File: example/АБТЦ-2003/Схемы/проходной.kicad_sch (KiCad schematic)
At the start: 27 parts

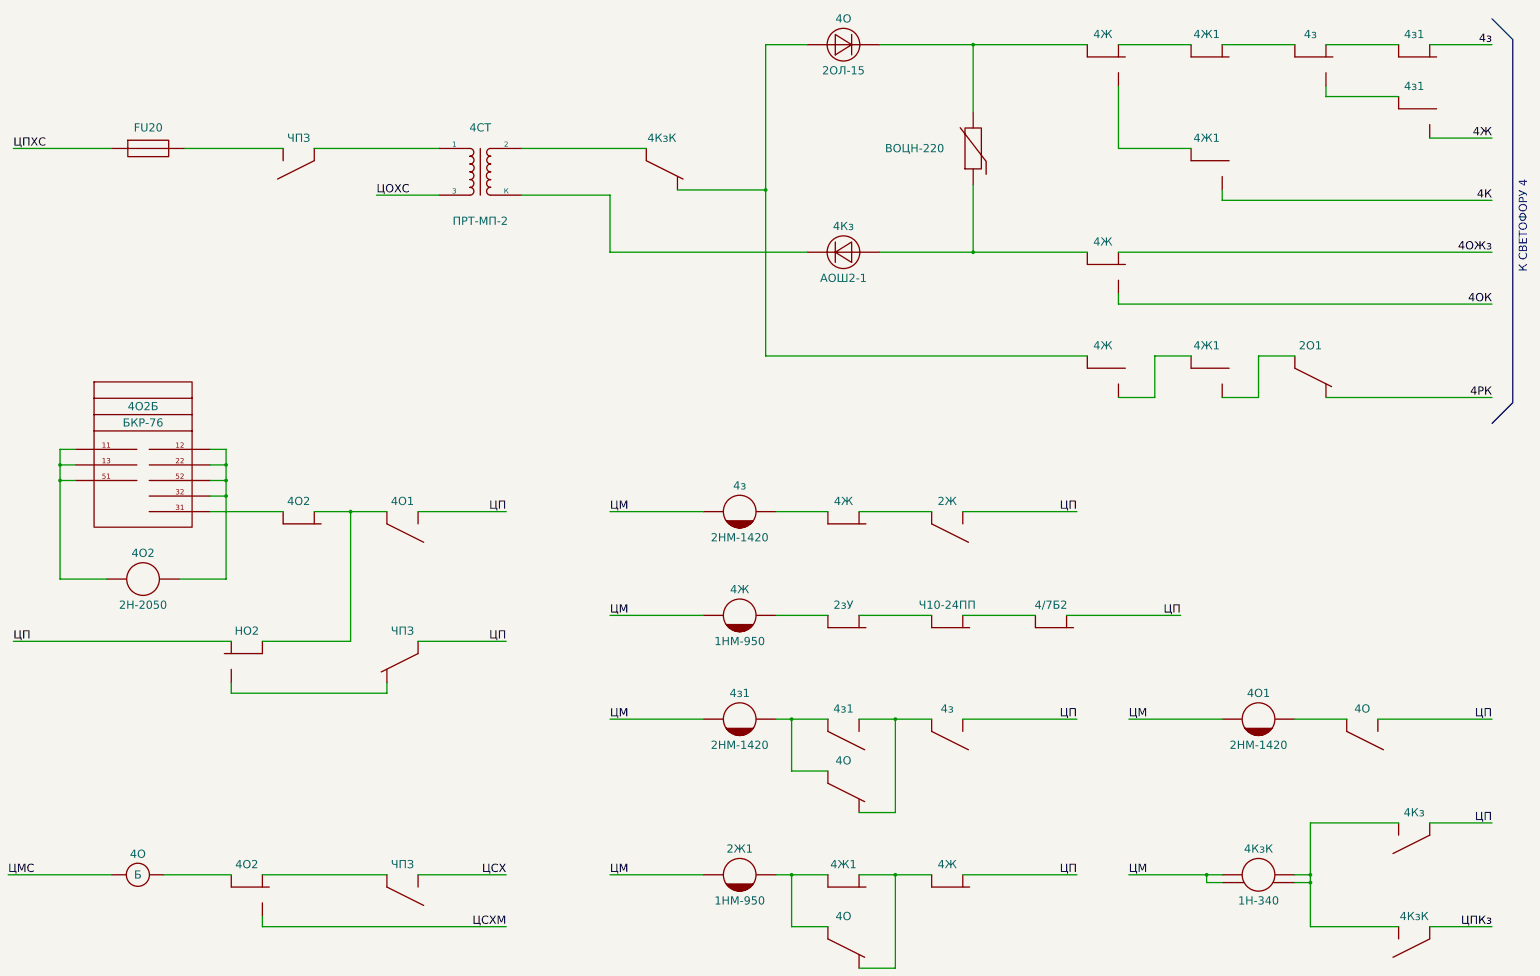
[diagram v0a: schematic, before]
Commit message: Шаблон АБТЦ обновлен
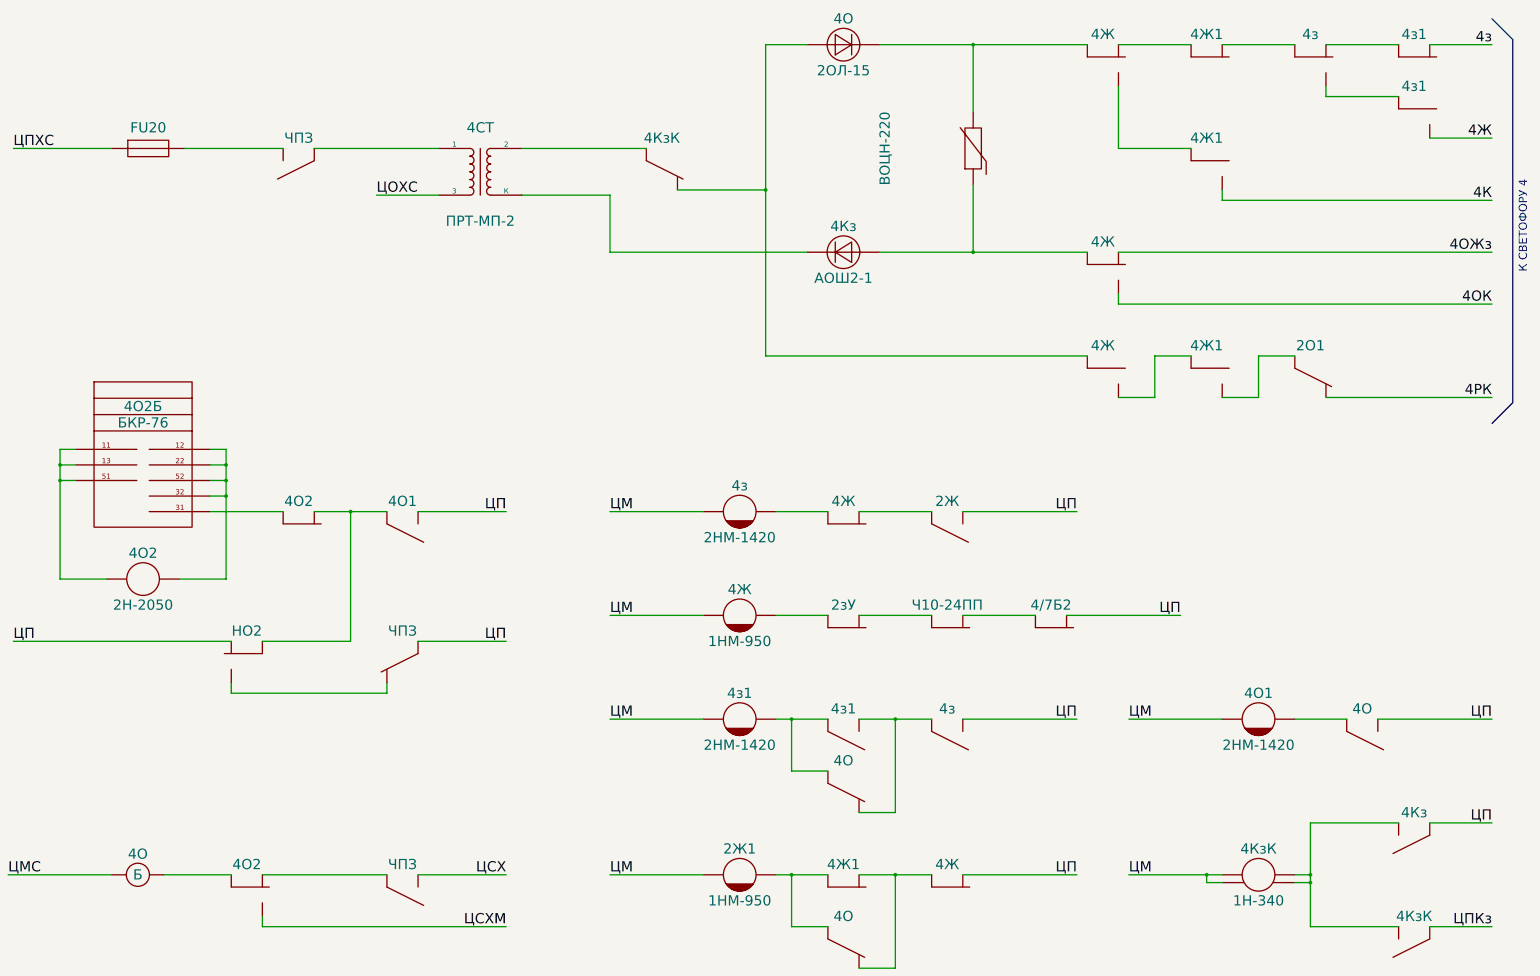
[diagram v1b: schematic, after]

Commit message: Обновление примера
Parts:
- Н11, Н111, Н1111, Н11111, Н1111111, Н11111111, Н111111111, Н1111111111, Н1111111112, Н111111112: symbol SCB_Relay:Контакт_нейтрального_якоря_НЗ -> SCB_Legacy:Контакт_нейтрального_якоря_НЗ_бн
- Н111, Н1111, Н11111, Н111111, Н1111111, Н11111111, Н111111111, Н1111111111, Н11111111111, Н12: symbol SCB_Relay:Контакт_нейтрального_якоря -> SCB_Legacy:Контакт_нейтрального_якоря_бн
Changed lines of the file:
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@@
 (kicad_sch
-	(version 20231120)
+	(version 20250114)
 	(generator "eeschema")
-	(generator_version "8.0")
+	(generator_version "9.0")
 	(paper "A3")
 	(title_block
@@
 		(comment 9 "Схема включения огней светофора 2")
 	)
+	(text "К СВЕТОФОРУ 4"
+		(exclude_from_sim no)
+		(at 401.32 82.55 90)
+		(effects
+			(font
+				(size 2 2)
+			)
+		)
+	)
 	(junction
 		(at 83.82 148.59)
@@
 		)
 	)
-	(text "К СВЕТОФОРУ 4"
-		(exclude_from_sim no)
-		(at 401.32 82.55 90)
-		(effects
-			(font
-				(size 2 2)
-			)
-		)
-	)
 	(label "ЦПКз"
 		(at 393.7 254 180)
@@
 	)
 	(symbol
-		(lib_id "SCB_Relay:Контакт_нейтрального_якоря_НЗ")
+		(lib_name "Контакт_нейтрального_якоря_НЗ_бн_9")
+		(lib_id "SCB_Legacy:Контакт_нейтрального_якоря_НЗ_бн")
 		(at 323.85 63.5 0)
 		(unit 2)
@@
 	)
 	(symbol
-		(lib_id "SCB_Relay:Контакт_нейтрального_якоря")
+		(lib_name "Контакт_нейтрального_якоря_бн_11")
+		(lib_id "SCB_Legacy:Контакт_нейтрального_якоря_бн")
 		(at 349.25 114.3 0)
 		(unit 2)
@@
 	)
 	(symbol
-		(lib_name "SCB_Relay:Контакт_нейтрального_якоря_НЗ")
-		(lib_id "SCB_Relay:Контакт_нейтрального_якоря_НЗ")
+		(lib_name "Контакт_нейтрального_якоря_НЗ_бн_2")
+		(lib_id "SCB_Legacy:Контакт_нейтрального_якоря_НЗ_бн")
 		(at 260.35 241.3 0)
 		(unit 3)
@@
 	)
 	(symbol
-		(lib_name "SCB_Relay:Контакт_нейтрального_якоря")
-		(lib_id "SCB_Relay:Контакт_нейтрального_якоря")
+		(lib_name "Контакт_нейтрального_якоря_бн_4")
+		(lib_id "SCB_Legacy:Контакт_нейтрального_якоря_бн")
 		(at 361.95 203.2 0)
 		(unit 3)
@@
 	)
 	(symbol
-		(lib_name "SCB_Relay:Контакт_нейтрального_якоря")
-		(lib_id "SCB_Relay:Контакт_нейтрального_якоря")
+		(lib_name "Контакт_нейтрального_якоря_бн_12")
+		(lib_id "SCB_Legacy:Контакт_нейтрального_якоря_бн")
 		(at 260.35 152.4 0)
 		(unit 3)
@@
 	)
 	(symbol
-		(lib_name "SCB_Relay:Контакт_нейтрального_якоря")
-		(lib_id "SCB_Relay:Контакт_нейтрального_якоря")
+		(lib_id "SCB_Legacy:Контакт_нейтрального_якоря_бн")
 		(at 374.65 254 0)
 		(mirror y)
@@
 	)
 	(symbol
-		(lib_name "SCB_Relay:Контакт_нейтрального_якоря_НЗ")
-		(lib_id "SCB_Relay:Контакт_нейтрального_якоря_НЗ")
+		(lib_id "SCB_Legacy:Контакт_нейтрального_якоря_НЗ_бн")
 		(at 260.35 177.8 0)
 		(unit 3)
@@
 	)
 	(symbol
-		(lib_name "SCB_Relay:Контакт_нейтрального_якоря_НЗ")
-		(lib_id "SCB_Relay:Контакт_нейтрального_якоря_НЗ")
+		(lib_name "Контакт_нейтрального_якоря_НЗ_бн_3")
+		(lib_id "SCB_Legacy:Контакт_нейтрального_якоря_НЗ_бн")
 		(at 234.95 177.8 0)
 		(unit 3)
@@
 	)
 	(symbol
-		(lib_name "SCB_Relay:Контакт_нейтрального_якоря")
-		(lib_id "SCB_Relay:Контакт_нейтрального_якоря")
+		(lib_name "Контакт_нейтрального_якоря_бн_5")
+		(lib_id "SCB_Legacy:Контакт_нейтрального_якоря_бн")
 		(at 234.95 215.9 0)
 		(unit 2)
@@
 	)
 	(symbol
-		(lib_name "SCB_Relay:Контакт_нейтрального_якоря")
-		(lib_id "SCB_Relay:Контакт_нейтрального_якоря")
+		(lib_name "Контакт_нейтрального_якоря_бн_7")
+		(lib_id "SCB_Legacy:Контакт_нейтрального_якоря_бн")
 		(at 127 241.3 0)
 		(unit 3)
@@
 	)
 	(symbol
-		(lib_name "SCB_Relay:Контакт_нейтрального_якоря_НЗ")
-		(lib_id "SCB_Relay:Контакт_нейтрального_якоря_НЗ")
+		(lib_name "Контакт_нейтрального_якоря_НЗ_бн_1")
+		(lib_id "SCB_Legacy:Контакт_нейтрального_якоря_НЗ_бн")
 		(at 234.95 152.4 0)
 		(unit 3)
@@
 	)
 	(symbol
-		(lib_name "SCB_Relay:Контакт_нейтрального_якоря")
-		(lib_id "SCB_Relay:Контакт_нейтрального_якоря")
+		(lib_name "Контакт_нейтрального_якоря_бн_3")
+		(lib_id "SCB_Legacy:Контакт_нейтрального_якоря_бн")
 		(at 234.95 254 0)
 		(unit 2)
@@
 	)
 	(symbol
-		(lib_name "SCB_Relay:Контакт_нейтрального_якоря_НЗ")
-		(lib_id "SCB_Relay:Контакт_нейтрального_якоря_НЗ")
+		(lib_name "Контакт_нейтрального_якоря_НЗ_бн_13")
+		(lib_id "SCB_Legacy:Контакт_нейтрального_якоря_НЗ_бн")
 		(at 101.6 152.4 0)
 		(unit 3)
@@
 	)
 	(symbol
-		(lib_name "SCB_Relay:Контакт_нейтрального_якоря")
-		(lib_id "SCB_Relay:Контакт_нейтрального_якоря")
+		(lib_name "Контакт_нейтрального_якоря_бн_13")
+		(lib_id "SCB_Legacy:Контакт_нейтрального_якоря_бн")
 		(at 234.95 203.2 0)
 		(unit 3)
@@
 	)
 	(symbol
-		(lib_name "SCB_Relay:Контакт_нейтрального_якоря")
-		(lib_id "SCB_Relay:Контакт_нейтрального_якоря")
+		(lib_name "Контакт_нейтрального_якоря_бн_8")
+		(lib_id "SCB_Legacy:Контакт_нейтрального_якоря_бн")
 		(at 260.35 203.2 0)
 		(unit 3)
@@
 	)
 	(symbol
-		(lib_name "SCB_Relay:Контакт_нейтрального_якоря_НЗ")
-		(lib_id "SCB_Relay:Контакт_нейтрального_якоря_НЗ")
+		(lib_name "Контакт_нейтрального_якоря_НЗ_бн_16")
+		(lib_id "SCB_Legacy:Контакт_нейтрального_якоря_НЗ_бн")
 		(at 323.85 38.1 0)
 		(unit 3)
@@
 	)
 	(symbol
-		(lib_name "SCB_Relay:Контакт_нейтрального_якоря_НЗ")
-		(lib_id "SCB_Relay:Контакт_нейтрального_якоря_НЗ")
+		(lib_name "Контакт_нейтрального_якоря_НЗ_бн_6")
+		(lib_id "SCB_Legacy:Контакт_нейтрального_якоря_НЗ_бн")
 		(at 374.65 50.8 0)
 		(unit 2)
@@
 	)
 	(symbol
-		(lib_name "SCB_Relay:Контакт_нейтрального_якоря_НЗ")
-		(lib_id "SCB_Relay:Контакт_нейтрального_якоря_НЗ")
+		(lib_name "Контакт_нейтрального_якоря_НЗ_бн_14")
+		(lib_id "SCB_Legacy:Контакт_нейтрального_якоря_НЗ_бн")
 		(at 298.45 114.3 0)
 		(unit 2)
@@
 	)
 	(symbol
-		(lib_name "SCB_Relay:Контакт_нейтрального_якоря")
-		(lib_id "SCB_Relay:Контакт_нейтрального_якоря")
+		(lib_name "Контакт_нейтрального_якоря_бн_6")
+		(lib_id "SCB_Legacy:Контакт_нейтрального_якоря_бн")
 		(at 374.65 228.6 0)
 		(mirror y)
@@
 	)
 	(symbol
-		(lib_name "SCB_Relay:Контакт_нейтрального_якоря")
-		(lib_id "SCB_Relay:Контакт_нейтрального_якоря")
+		(lib_name "Контакт_нейтрального_якоря_бн_10")
+		(lib_id "SCB_Legacy:Контакт_нейтрального_якоря_бн")
 		(at 190.5 63.5 0)
 		(unit 2)
@@
 	)
 	(symbol
-		(lib_name "SCB_Relay:Контакт_нейтрального_якоря")
-		(lib_id "SCB_Relay:Контакт_нейтрального_якоря")
+		(lib_name "Контакт_нейтрального_якоря_бн_1")
+		(lib_id "SCB_Legacy:Контакт_нейтрального_якоря_бн")
 		(at 101.6 63.5 0)
 		(mirror y)
@@
 	)
 	(symbol
-		(lib_name "SCB_Relay:Контакт_нейтрального_якоря_НЗ")
-		(lib_id "SCB_Relay:Контакт_нейтрального_якоря_НЗ")
+		(lib_name "Контакт_нейтрального_якоря_НЗ_бн_17")
+		(lib_id "SCB_Legacy:Контакт_нейтрального_якоря_НЗ_бн")
 		(at 349.25 38.1 0)
 		(unit 1)
@@
 	)
 	(symbol
-		(lib_name "SCB_Relay:Контакт_нейтрального_якоря")
-		(lib_id "SCB_Relay:Контакт_нейтрального_якоря")
+		(lib_name "Контакт_нейтрального_якоря_бн_9")
+		(lib_id "SCB_Legacy:Контакт_нейтрального_якоря_бн")
 		(at 127 184.15 0)
 		(mirror y)
@@
 	)
 	(symbol
-		(lib_name "SCB_Relay:Контакт_нейтрального_якоря_НЗ")
-		(lib_id "SCB_Relay:Контакт_нейтрального_якоря_НЗ")
+		(lib_name "Контакт_нейтрального_якоря_НЗ_бн_10")
+		(lib_id "SCB_Legacy:Контакт_нейтрального_якоря_НЗ_бн")
 		(at 88.9 184.15 0)
 		(mirror y)
@@
 	)
 	(symbol
-		(lib_name "SCB_Relay:Контакт_нейтрального_якоря_НЗ")
-		(lib_id "SCB_Relay:Контакт_нейтрального_якоря_НЗ")
+		(lib_name "Контакт_нейтрального_якоря_НЗ_бн_7")
+		(lib_id "SCB_Legacy:Контакт_нейтрального_якоря_НЗ_бн")
 		(at 285.75 177.8 0)
 		(unit 3)
@@
 	)
 	(symbol
-		(lib_name "SCB_Relay:Контакт_нейтрального_якоря_НЗ")
-		(lib_id "SCB_Relay:Контакт_нейтрального_якоря_НЗ")
+		(lib_name "Контакт_нейтрального_якоря_НЗ_бн_11")
+		(lib_id "SCB_Legacy:Контакт_нейтрального_якоря_НЗ_бн")
 		(at 298.45 88.9 0)
 		(unit 1)
@@
 	)
 	(symbol
-		(lib_name "SCB_Relay:Контакт_нейтрального_якоря_НЗ")
-		(lib_id "SCB_Relay:Контакт_нейтрального_якоря_НЗ")
+		(lib_name "Контакт_нейтрального_якоря_НЗ_бн_5")
+		(lib_id "SCB_Legacy:Контакт_нейтрального_якоря_НЗ_бн")
 		(at 323.85 114.3 0)
 		(unit 2)
@@
 	)
 	(symbol
-		(lib_name "SCB_Relay:Контакт_нейтрального_якоря")
-		(lib_id "SCB_Relay:Контакт_нейтрального_якоря")
+		(lib_name "Контакт_нейтрального_якоря_бн_2")
+		(lib_id "SCB_Legacy:Контакт_нейтрального_якоря_бн")
 		(at 127 152.4 0)
 		(unit 3)
@@
 	)
 	(symbol
-		(lib_name "SCB_Relay:Контакт_нейтрального_якоря_НЗ")
-		(lib_id "SCB_Relay:Контакт_нейтрального_якоря_НЗ")
+		(lib_name "Контакт_нейтрального_якоря_НЗ_бн_8")
+		(lib_id "SCB_Legacy:Контакт_нейтрального_якоря_НЗ_бн")
 		(at 234.95 241.3 0)
 		(unit 3)
@@
 	)
 	(symbol
-		(lib_name "SCB_Relay:Контакт_нейтрального_якоря_НЗ")
-		(lib_id "SCB_Relay:Контакт_нейтрального_якоря_НЗ")
+		(lib_name "Контакт_нейтрального_якоря_НЗ_бн_15")
+		(lib_id "SCB_Legacy:Контакт_нейтрального_якоря_НЗ_бн")
 		(at 374.65 38.1 0)
 		(unit 3)
@@
 	)
 	(symbol
-		(lib_name "SCB_Relay:Контакт_нейтрального_якоря_НЗ")
-		(lib_id "SCB_Relay:Контакт_нейтрального_якоря_НЗ")
+		(lib_name "Контакт_нейтрального_якоря_НЗ_бн_4")
+		(lib_id "SCB_Legacy:Контакт_нейтрального_якоря_НЗ_бн")
 		(at 298.45 38.1 0)
 		(unit 1)
@@
 	)
 	(symbol
-		(lib_name "SCB_Relay:Контакт_нейтрального_якоря_НЗ")
-		(lib_id "SCB_Relay:Контакт_нейтрального_якоря_НЗ")
+		(lib_name "Контакт_нейтрального_якоря_НЗ_бн_12")
+		(lib_id "SCB_Legacy:Контакт_нейтрального_якоря_НЗ_бн")
 		(at 88.9 241.3 0)
 		(unit 1)
